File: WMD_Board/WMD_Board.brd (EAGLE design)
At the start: 65 x 45 mm, 45 parts, among them J1 EMPCB.SMAFSTJ.B.HT, U1 STM32L053C8T6, U2 BSS138, U3 RFM69HCW, U4 BSS138, Y2 ABS06-107-32.768KHZ-T

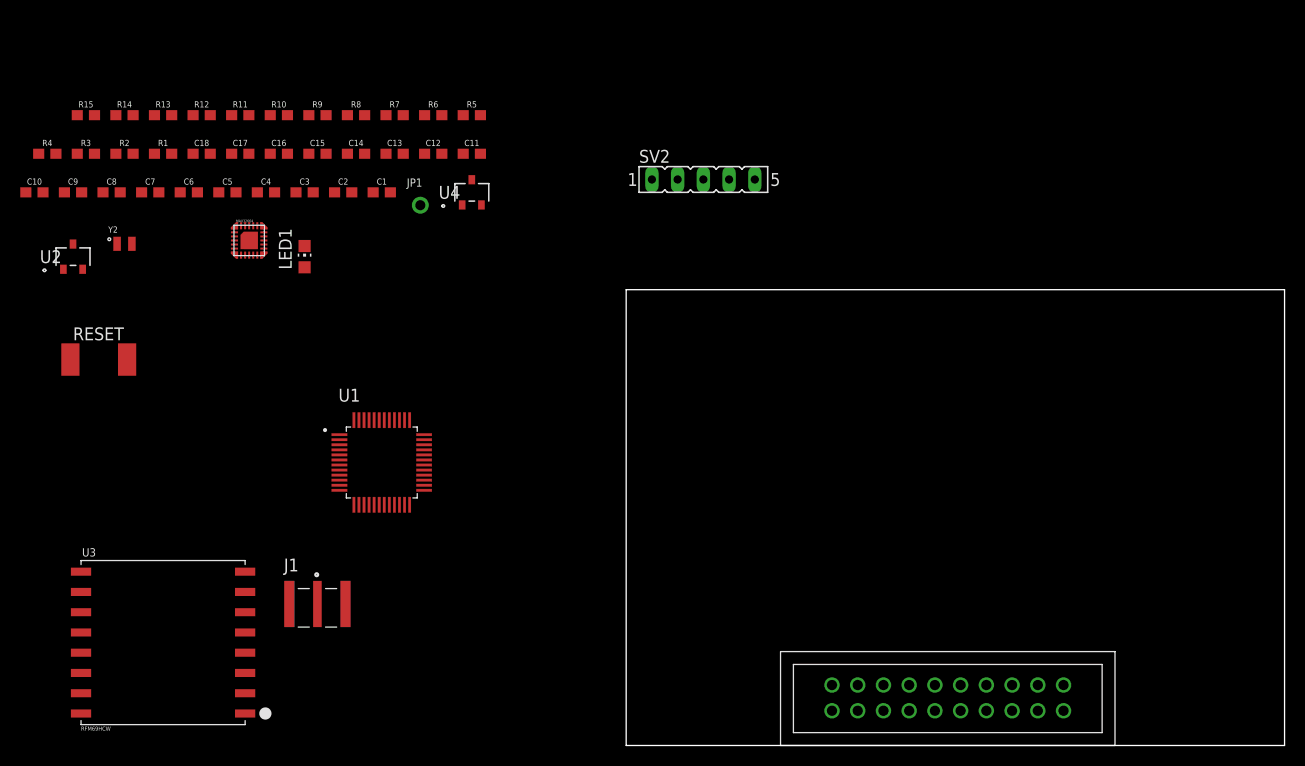
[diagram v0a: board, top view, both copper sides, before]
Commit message: More Schematic Work
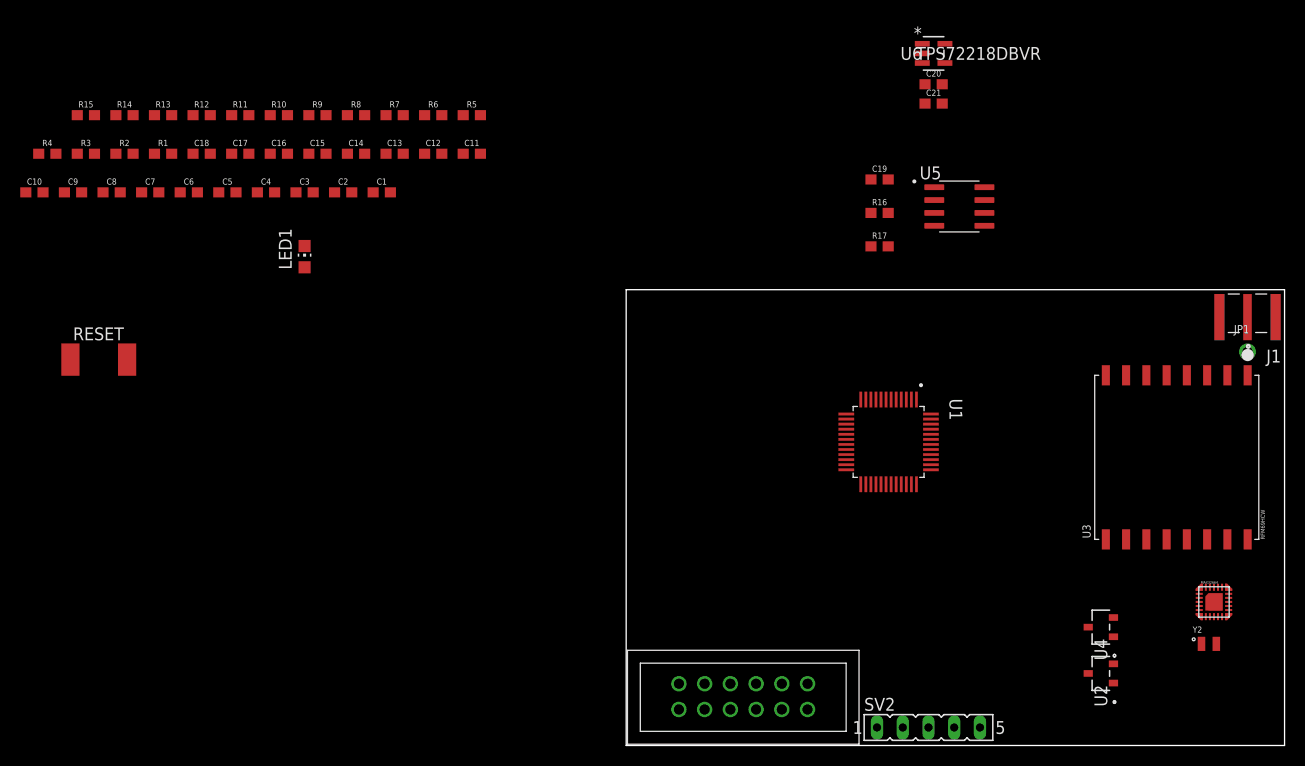
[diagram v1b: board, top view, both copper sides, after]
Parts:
- added C19, C20, C21: 0.1uF, SparkFun-Capacitors:0603
- added R16, R17: 4.7k, SparkFun-Resistors:0603
- added U5: M24512-DRMN8TP/K, M24512_EEPROM:SOIC127P600X175-8N
- added U6: TPS72218DBVR, TPS72218DBVR_LDO:DBV5
- U$20: value TS_DR_10 -> TS_DR_6; device TST_Connnector:TST_DR_10 -> TST_Connnector:TST_DR_6
- moved Y2 114.1 mm to (57.5, 10.0)
- moved U2 109.5 mm to (46.9, 7.11), turned to 90 degrees
- moved U3 101.7 mm to (54.4, 28.4), turned to 90 degrees
- moved U$10 101.7 mm to (55.9, 12.6)
- moved J1 96.1 mm to (61.3, 42.3), turned to 180 degrees
- moved JP1 82.9 mm to (61.3, 38.9)
- moved U4 75.5 mm to (46.9, 11.7), turned to 90 degrees
- moved SV2 58.5 mm to (29.8, 1.78)
- moved U1 50.1 mm to (25.9, 30.0), turned to 270 degrees
- moved U$20 15.1 mm to (0.13, 0.13)
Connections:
- net CS renamed LORA_CS
- net RST renamed LORA_RESET
- net SPI1_MISO renamed LORA_MISO
- net SPI1_MOSI renamed LORA_MOSI
- net SPI1_SCK renamed LORA_SCK
- removed net BTN_1_1: R7.1, R8.2, U$20.11
- removed net BTN_2_1: R10.1, R11.2, U$20.12
- removed net BTN_3_1: R12.1, R13.2, U$20.13
- removed net BTN_4_1: R14.1, R15.2, U$20.14
- removed net DIO5: U3.15P
- removed net GPS_RX: U1.22
- removed net GPS_TX: U1.21
- removed net MFIO: U$10.MFIO@1, U$10.MFIO@2
- removed net N$2: R2.2, U1.25
- removed net RSTN: C14.1, U$10.RSTN
- new net BTN1_OUT: R7.1, R8.2, U$20.1
- new net BTN2_OUT: R10.1, R11.2, U$20.2
- new net BTN3_OUT: R12.1, R13.2, U$20.7
- new net BTN4_OUT: R14.1, R15.2, U$20.8
- new net HR_MFIO: U$10.MFIO@1, U$10.MFIO@2, U1.40
- new net HR_RESET: C14.1, U$10.RSTN, U1.41
- new net LORA_DIO5: U1.19, U3.15P
- new net N$1: R2.2, U1.39
- new net OLED_CS: U$20.3, U1.25
- new net OLED_DC: U$20.5, U1.27
- new net OLED_MOSI: U$20.6, U1.28
- new net OLED_RESET: U$20.12, U1.29
- new net OLED_SCK: U$20.4, U1.26
- new net WC_EEPROM: U1.46, U5.7
- net 1.8V: now also C20.1, U6.5
- net 3.3V: now also C19.1, C21.1, R16.1, R17.1, U$20.11, U5.8, U6.1, U6.3
- net BTN1: now also U1.10
- net BTN2: now also U1.11
- net BTN3: now also U1.12
- net BTN4: now also U1.13
- net DIO0: no longer U1.19
- net GND: now also C19.2, C20.2, C21.2, U$20.10, U$20.9, U5.1, U5.2, U5.3, U5.4, U6.2; no longer U$20.1, U$20.2, U$20.3, U$20.4
- net SCL_EEPROM: now also R17.2, U1.21, U5.6; no longer U1.26
- net SDA_EEPROM: now also R16.2, U1.22, U5.5; no longer U1.27

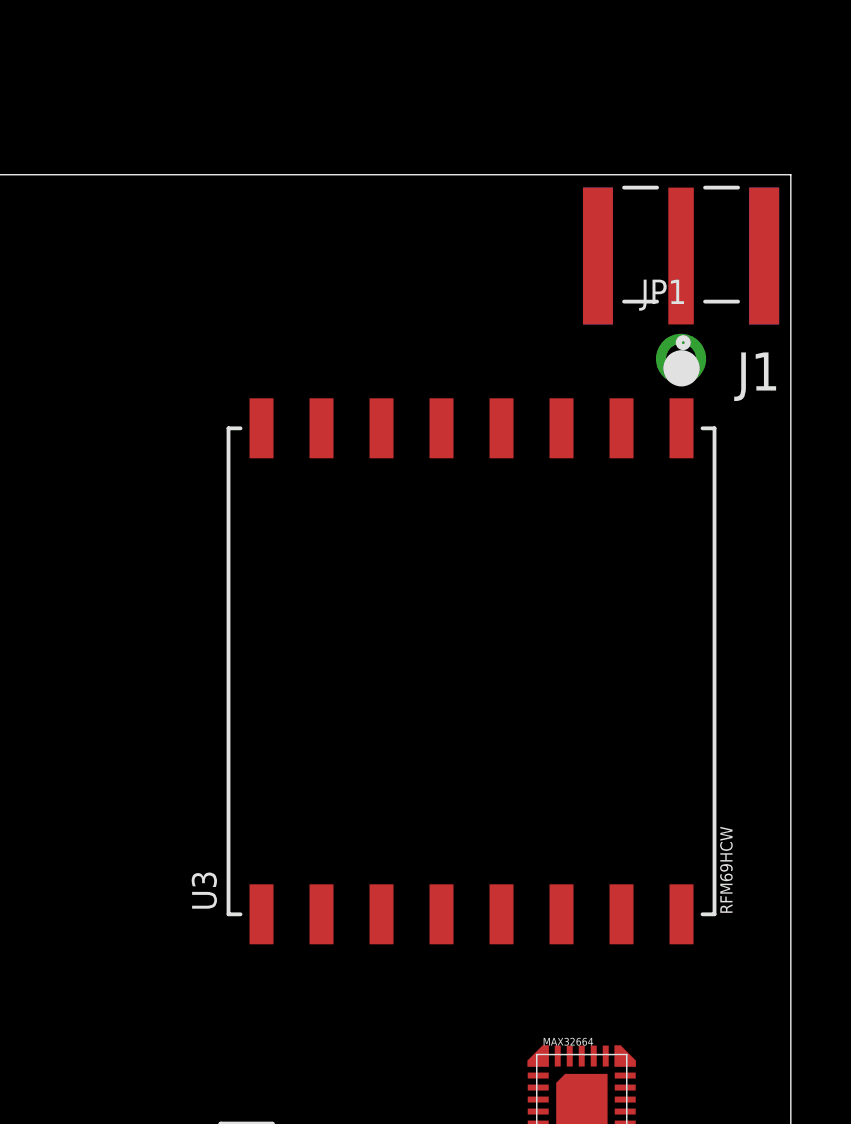
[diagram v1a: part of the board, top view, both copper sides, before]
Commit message: stuff
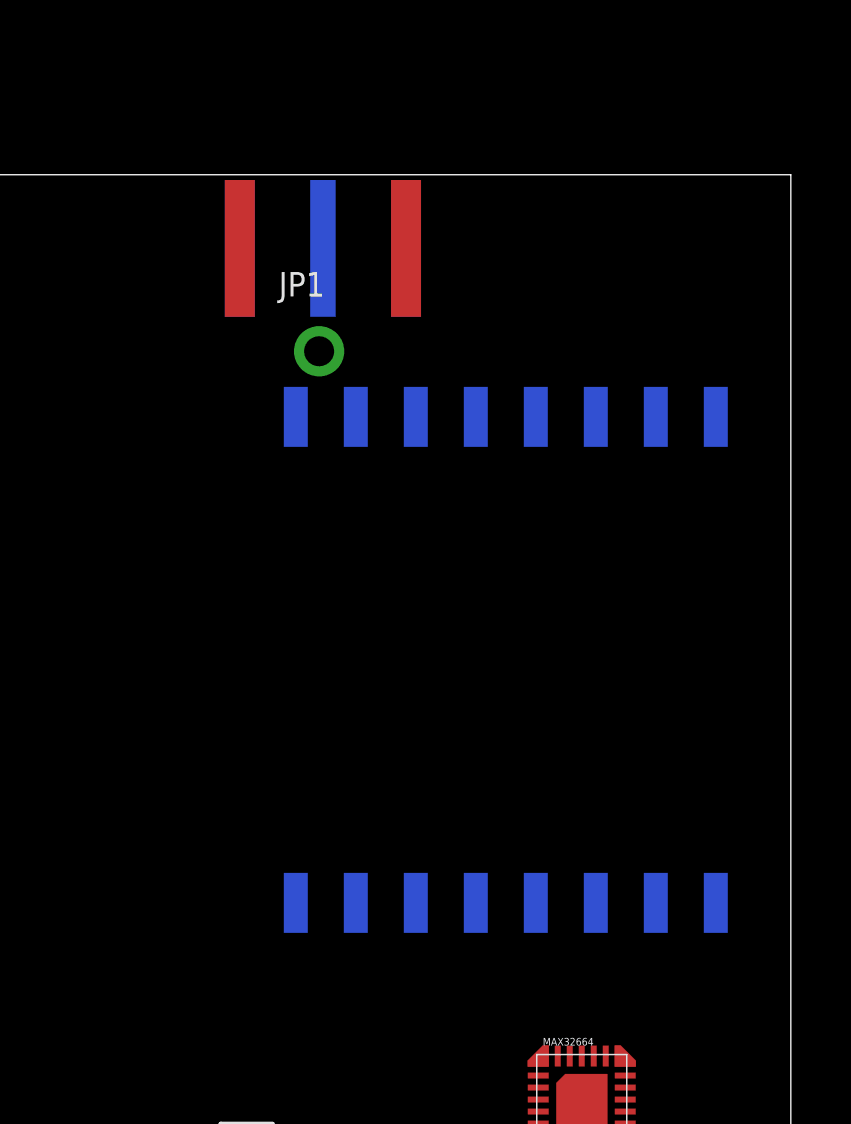
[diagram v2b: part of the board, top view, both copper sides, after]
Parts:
- moved JP1 12.1 mm to (49.3, 39.1)
- moved J1 11.9 mm to (49.4, 42.5), flipped to the bottom
- moved U3 1.20 mm to (55.5, 28.8), flipped to the bottom
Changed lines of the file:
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@@
 <attribute name="PROD_ID" value="CAP-00810" x="-54.61" y="54.61" size="1.778" layer="27" display="off"/>
 </element>
-<element name="J1" library="EMPCB.SMAFSTJ.B.HT" package="TAOGLAS_EMPCB.SMAFSTJ.B.HT" value="EMPCB.SMAFSTJ.B.HT" x="61.341" y="42.291" rot="R180">
-<attribute name="DESCRIPTION" value=" SMA Connector Jack, Female Socket 50Ohm Board Edge, End Launch Solder " x="61.341" y="42.291" size="1.778" layer="27" rot="R180" display="off"/>
-<attribute name="DIGI-KEY_PART_NUMBER" value="931-1175-ND" x="61.341" y="42.291" size="1.778" layer="27" rot="R180" display="off"/>
-<attribute name="DIGI-KEY_PURCHASE_URL" value="https://www.digikey.com/product-detail/en/taoglas-limited/EMPCB.SMAFSTJ.B.HT/931-1175-ND/3522337?utm_source=snapeda&amp;utm_medium=aggregator&amp;utm_campaign=symbol" x="61.341" y="42.291" size="1.778" layer="27" rot="R180" display="off"/>
-<attribute name="MF" value="Taoglas Limited" x="61.341" y="42.291" size="1.778" layer="27" rot="R180" display="off"/>
-<attribute name="MP" value="EMPCB.SMAFSTJ.B.HT" x="61.341" y="42.291" size="1.778" layer="27" rot="R180" display="off"/>
-<attribute name="PACKAGE" value="None" x="61.341" y="42.291" size="1.778" layer="27" rot="R180" display="off"/>
-</element>
-<element name="JP1" library="microbuilder" package="1X01_ROUND" value="" x="61.341" y="38.862"/>
+<element name="J1" library="EMPCB.SMAFSTJ.B.HT" package="TAOGLAS_EMPCB.SMAFSTJ.B.HT" value="EMPCB.SMAFSTJ.B.HT" x="49.403" y="42.545" rot="MR180">
+<attribute name="DESCRIPTION" value=" SMA Connector Jack, Female Socket 50Ohm Board Edge, End Launch Solder " x="49.403" y="42.545" size="1.778" layer="28" rot="MR180" display="off"/>
+<attribute name="DIGI-KEY_PART_NUMBER" value="931-1175-ND" x="49.403" y="42.545" size="1.778" layer="28" rot="MR180" display="off"/>
+<attribute name="DIGI-KEY_PURCHASE_URL" value="https://www.digikey.com/product-detail/en/taoglas-limited/EMPCB.SMAFSTJ.B.HT/931-1175-ND/3522337?utm_source=snapeda&amp;utm_medium=aggregator&amp;utm_campaign=symbol" x="49.403" y="42.545" size="1.778" layer="28" rot="MR180" display="off"/>
+<attribute name="MF" value="Taoglas Limited" x="49.403" y="42.545" size="1.778" layer="28" rot="MR180" display="off"/>
+<attribute name="MP" value="EMPCB.SMAFSTJ.B.HT" x="49.403" y="42.545" size="1.778" layer="28" rot="MR180" display="off"/>
+<attribute name="PACKAGE" value="None" x="49.403" y="42.545" size="1.778" layer="28" rot="MR180" display="off"/>
+</element>
+<element name="JP1" library="microbuilder" package="1X01_ROUND" value="" x="49.276" y="39.116"/>
 <element name="LED1" library="led" library_urn="urn:adsk.eagle:library:259" package="CHIP-LED0805" package3d_urn="urn:adsk.eagle:package:15818/2" value="" x="-31.75" y="48.26">
 <attribute name="POPULARITY" value="68" x="-31.75" y="48.26" size="1.778" layer="27" display="off"/>
@@
 <attribute name="VENDOR" value="Fairchild Semiconductor" x="46.863" y="7.112" size="1.778" layer="27" rot="R90" display="off"/>
 </element>
-<element name="U3" library="microbuilder" package="RFMHCW_SMT" value="RFM69HCW" x="54.356" y="28.448" rot="R90"/>
+<element name="U3" library="microbuilder" package="RFMHCW_SMT" value="RFM69HCW" x="55.499" y="28.829" rot="MR90"/>
 <element name="U4" library="BSS138" package="SOT-23-3L" value="BSS138" x="46.863" y="11.684" rot="R90">
 <attribute name="MANUFACTURER_PART_NUMBER" value="BSS138" x="46.863" y="11.684" size="1.778" layer="27" rot="R90" display="off"/>
@@
 <contactref element="C21" pad="2"/>
 <contactref element="U6" pad="2"/>
-<wire x1="64.111" y1="42.291" x2="64.111" y2="42.291" width="0" layer="19" extent="1-16"/>
-<wire x1="58.571" y1="42.291" x2="64.111" y2="42.291" width="0" layer="19" extent="1-1"/>
-<wire x1="58.571" y1="42.291" x2="58.571" y2="42.291" width="0" layer="19" extent="1-16"/>
-<wire x1="59.356" y1="36.548" x2="58.571" y2="42.291" width="0" layer="19" extent="1-1"/>
-<wire x1="61.356" y1="20.348" x2="59.356" y2="36.548" width="0" layer="19" extent="1-1"/>
-<wire x1="58.18" y1="14.173" x2="61.356" y2="20.348" width="0" layer="19" extent="1-1"/>
+<wire x1="52.173" y1="42.545" x2="46.633" y2="42.545" width="0" layer="19" extent="1-1"/>
+<wire x1="50.499" y1="36.929" x2="52.173" y2="42.545" width="0" layer="19" extent="1-1"/>
+<wire x1="48.499" y1="20.729" x2="50.499" y2="36.929" width="0" layer="19" extent="1-1"/>
+<wire x1="58.18" y1="14.173" x2="48.499" y2="20.729" width="0" layer="19" extent="1-1"/>
 <wire x1="58.03" y1="12.723" x2="58.18" y2="14.173" width="0" layer="19" extent="1-1"/>
 <wire x1="56.83" y1="12.623" x2="58.03" y2="12.723" width="0" layer="19" extent="1-1"/>
 <wire x1="56.58" y1="12.973" x2="56.83" y2="12.623" width="0" layer="19" extent="1-1"/>
-<wire x1="47.356" y1="20.348" x2="56.58" y2="12.973" width="0" layer="19" extent="1-1"/>
-<wire x1="28.158" y1="25.792" x2="47.356" y2="20.348" width="0" layer="19" extent="1-1"/>
+<wire x1="62.499" y1="20.729" x2="56.58" y2="12.973" width="0" layer="19" extent="1-1"/>
+<wire x1="28.158" y1="25.792" x2="62.499" y2="20.729" width="0" layer="19" extent="1-1"/>
 <wire x1="30.088" y1="32.222" x2="28.158" y2="25.792" width="0" layer="19" extent="1-1"/>
 <wire x1="25.158" y1="34.152" x2="30.088" y2="32.222" width="0" layer="19" extent="1-1"/>
@@
 <contactref element="U6" pad="1"/>
 <contactref element="C21" pad="1"/>
-<wire x1="30.088" y1="32.722" x2="53.356" y2="36.548" width="0" layer="19" extent="1-1"/>
+<wire x1="30.088" y1="32.722" x2="56.499" y2="36.929" width="0" layer="19" extent="1-1"/>
 <wire x1="24.658" y1="34.152" x2="30.088" y2="32.722" width="0" layer="19" extent="1-1"/>
 <wire x1="28.658" y1="25.792" x2="30.088" y2="32.722" width="0" layer="19" extent="1-1"/>
@@
 <contactref element="JP1" pad="1"/>
 <contactref element="J1" pad="1"/>
-<wire x1="61.341" y1="38.862" x2="61.341" y2="42.291" width="0" layer="19" extent="1-1"/>
-<wire x1="61.356" y1="36.548" x2="61.341" y2="38.862" width="0" layer="19" extent="1-1"/>
+<wire x1="49.276" y1="39.116" x2="49.403" y2="42.545" width="0" layer="19" extent="1-1"/>
+<wire x1="48.499" y1="36.929" x2="49.276" y2="39.116" width="0" layer="19" extent="1-1"/>
 </signal>
 <signal name="DIO3">
@@
 <contactref element="U3" pad="10P"/>
 <contactref element="U1" pad="16"/>
-<wire x1="21.728" y1="31.222" x2="49.356" y2="20.348" width="0" layer="19" extent="1-1"/>
+<wire x1="21.728" y1="31.222" x2="60.499" y2="20.729" width="0" layer="19" extent="1-1"/>
 </signal>
 <signal name="LORA_MOSI">
 <contactref element="U3" pad="11P"/>
 <contactref element="U1" pad="17"/>
-<wire x1="21.728" y1="30.722" x2="51.356" y2="20.348" width="0" layer="19" extent="1-1"/>
+<wire x1="21.728" y1="30.722" x2="58.499" y2="20.729" width="0" layer="19" extent="1-1"/>
 </signal>
 <signal name="LORA_SCK">
 <contactref element="U3" pad="12P"/>
 <contactref element="U1" pad="15"/>
-<wire x1="21.728" y1="31.722" x2="53.356" y2="20.348" width="0" layer="19" extent="1-1"/>
+<wire x1="21.728" y1="31.722" x2="56.499" y2="20.729" width="0" layer="19" extent="1-1"/>
 </signal>
 <signal name="LORA_CS">
 <contactref element="U3" pad="13P"/>
 <contactref element="U1" pad="14"/>
-<wire x1="21.728" y1="32.222" x2="55.356" y2="20.348" width="0" layer="19" extent="1-1"/>
+<wire x1="21.728" y1="32.222" x2="54.499" y2="20.729" width="0" layer="19" extent="1-1"/>
 </signal>
 <signal name="OLED_MOSI">
@@
 <contactref element="U1" pad="18"/>
 <contactref element="U3" pad="14P"/>
-<wire x1="21.728" y1="30.222" x2="57.356" y2="20.348" width="0" layer="19" extent="1-1"/>
+<wire x1="21.728" y1="30.222" x2="52.499" y2="20.729" width="0" layer="19" extent="1-1"/>
 </signal>
 <signal name="LORA_DIO5">
 <contactref element="U3" pad="15P"/>
 <contactref element="U1" pad="19"/>
-<wire x1="21.728" y1="29.722" x2="59.356" y2="20.348" width="0" layer="19" extent="1-1"/>
+<wire x1="21.728" y1="29.722" x2="50.499" y2="20.729" width="0" layer="19" extent="1-1"/>
 </signal>
 <signal name="N$1">
